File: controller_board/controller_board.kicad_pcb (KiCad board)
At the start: 2 copper layers, 62.6 x 67.2 mm, 9 parts, among them U1 NRF24L01_Breakout, U2 DEV-15583, U3 DM-OLED096-636, U4 TLV1117LV33DCYR

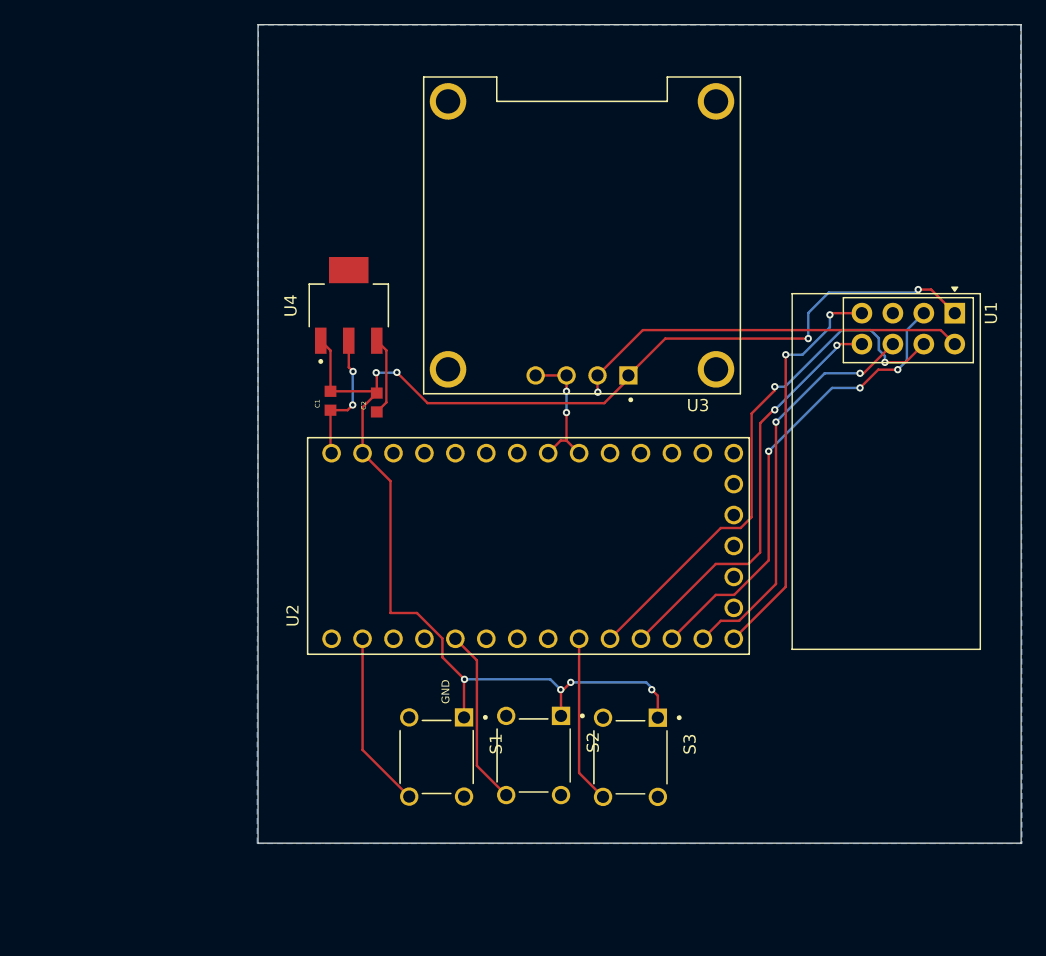
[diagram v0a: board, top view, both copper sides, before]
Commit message: adding gerber files
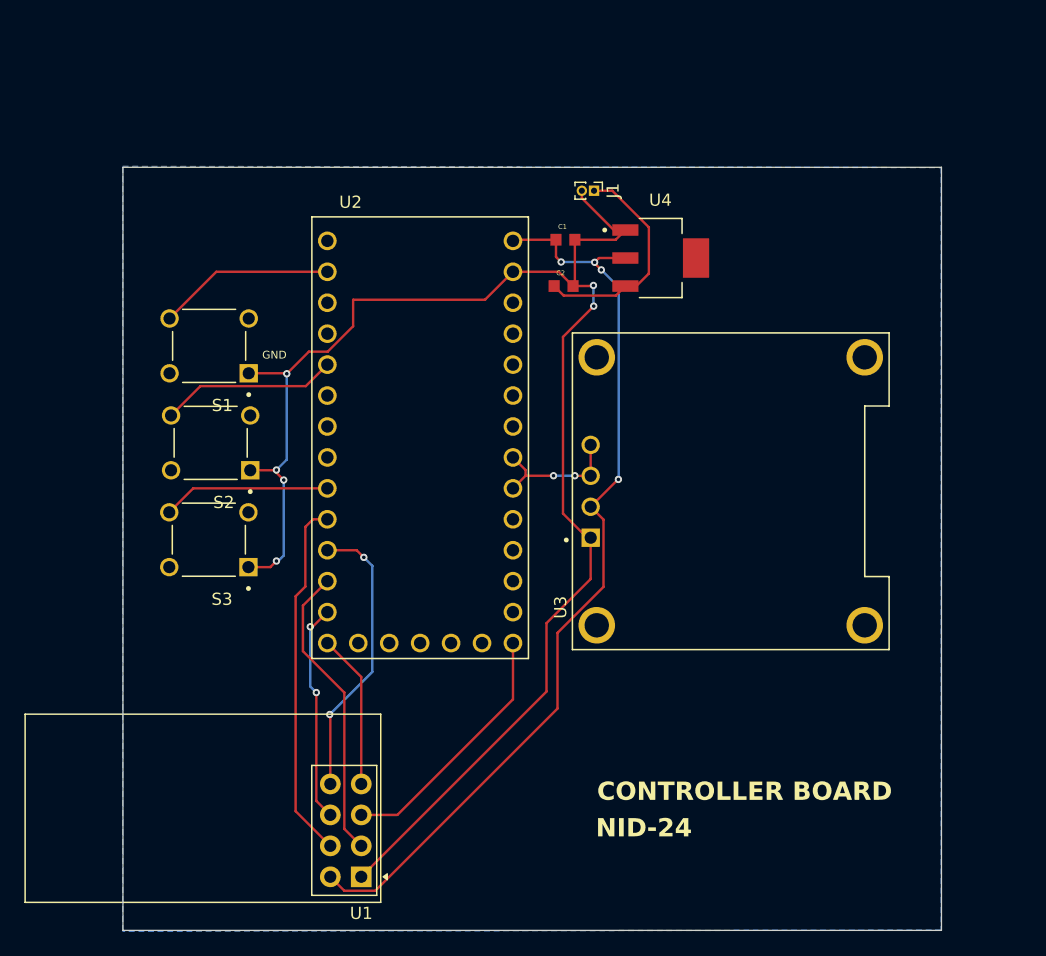
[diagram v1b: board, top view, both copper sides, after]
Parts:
- added J1: Conn_01x02_Pin, Connector_PinHeader_1.00mm:PinHeader_1x02_P1.00mm_Vertical, F.Cu at (138.3, 66.5)
- S1: value BTN_UP -> TS02-66-55-BK-100-LCR-D
- S2: value BTN_OK -> TS02-66-55-BK-100-LCR-D
- S3: value BTN DOWN -> TS02-66-55-BK-100-LCR-D
- moved U1 67.2 mm to (119.1, 122.8), turned to 180 degrees
- moved S3 39.0 mm to (106.6, 95.2), turned to 180 degrees
- moved S1 38.6 mm to (106.7, 79.2), turned to 180 degrees
- moved S2 36.9 mm to (106.8, 87.2), turned to 180 degrees
- moved U4 25.9 mm to (143.7, 72.0), turned to 0 degrees
- moved U3 24.3 mm to (149.5, 91.2), turned to 90 degrees
- moved C1 23.4 mm to (135.9, 70.5), turned to 0 degrees
- moved C2 18.1 mm to (135.8, 74.3), turned to 0 degrees
- moved U2 12.6 mm to (124.0, 87.1), turned to 0 degrees
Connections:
- C1 pad 1: Net-(U4-OUT_2) -> +3.3V
- U2 pad VIN: Net-(U4-OUT_2) -> +3.3V
- U4 pad 2: Net-(U4-OUT_2) -> +3.3V
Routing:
- net +3.3V: track 32.7 -> 76.8 mm, vias 1 -> 4
- net Net-(U1-SCK): track 0.00 -> 21.0 mm
- net Net-(U1-MISO): track 33.4 -> 12.7 mm, vias 2 -> 0
- net Net-(U1-MOSI): track 33.4 -> 18.0 mm
- net Net-(U1-~{CSN}): track 44.0 -> 29.8 mm, vias 2 -> 0
- net Net-(U1-CE): track 38.5 -> 24.5 mm, vias 3 -> 0
- net +5V: track 6.50 -> 18.4 mm
- net Net-(U4-OUT_2): track 11.0 -> 0.00 mm, vias 2 -> 0
- net Net-(U1-IRQ): track 34.5 -> 23.6 mm
- net GND: track 117.5 -> 126.7 mm, vias 8 -> 6
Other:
- board size 62.6 x 67.2 mm -> 67.2 x 62.7 mm
- board text added: "CONTROLLER BOARD"
- board text added: "NID-24"
